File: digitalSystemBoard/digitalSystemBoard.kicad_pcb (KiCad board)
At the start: 2 copper layers, 180 x 130 mm, 200 parts, among them J1 Barrel_Jack, J10 Conn_02x03_Odd_Even, J11 Conn_02x03_Odd_Even, J12 Conn_02x03_Odd_Even, J2 USB-B, J3 Conn_02x04_Odd_Even, J4 Conn_02x04_Odd_Even, J5 Conn_02x08_Odd_Even, J6 Conn_02x07_Odd_Even, J7 Conn_02x07_Odd_Even, J8 Conn_02x08_Odd_Even, J9 Conn_02x03_Odd_Even, Q10 BC847, Q11 BC847, Q12 BC847, Q13 BC847, Q14 BC847, Q15 BC847, Q16 BC847, Q17 BC847, Q2 BC847, Q3 BC847, Q4 BC847, Q5 BC847, Q6 BC847, Q7 BC847, Q8 BC847, Q9 BC847, SW1 SW_SPDT, SW9 ButtonFirst, U10 IO_Switch, U11 IO_Switch, U12 IO_Switch, U13 IO_Switch, U14 74LS04, U15 Potentiometer, U16 ATmega32U4-AU, U17 ICSP, U18 74LS165, U19 74HC595, U2 KCSA02-105, U20 74LS165, U21 74HC595, U3 KCSA02-105, U4 74LS47, U5 74LS47, U6 IO_Switch, U7 IO_Switch, U8 IO_Switch, U9 IO_Switch, Y1 16MHz

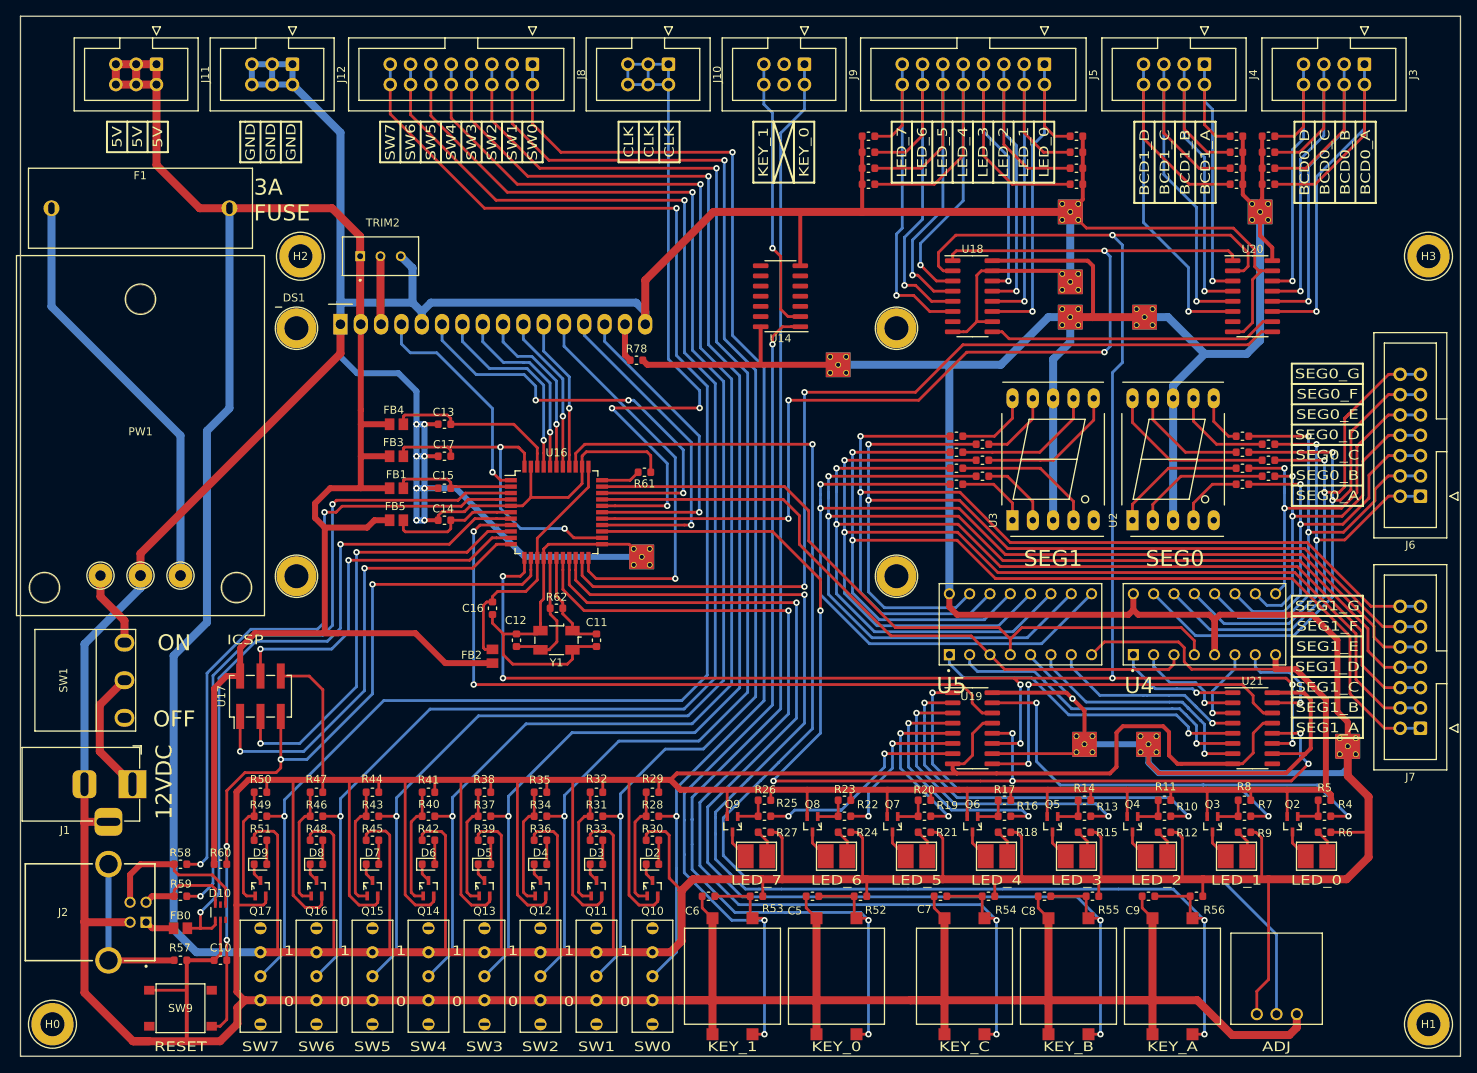
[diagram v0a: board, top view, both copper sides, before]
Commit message: Soldermask
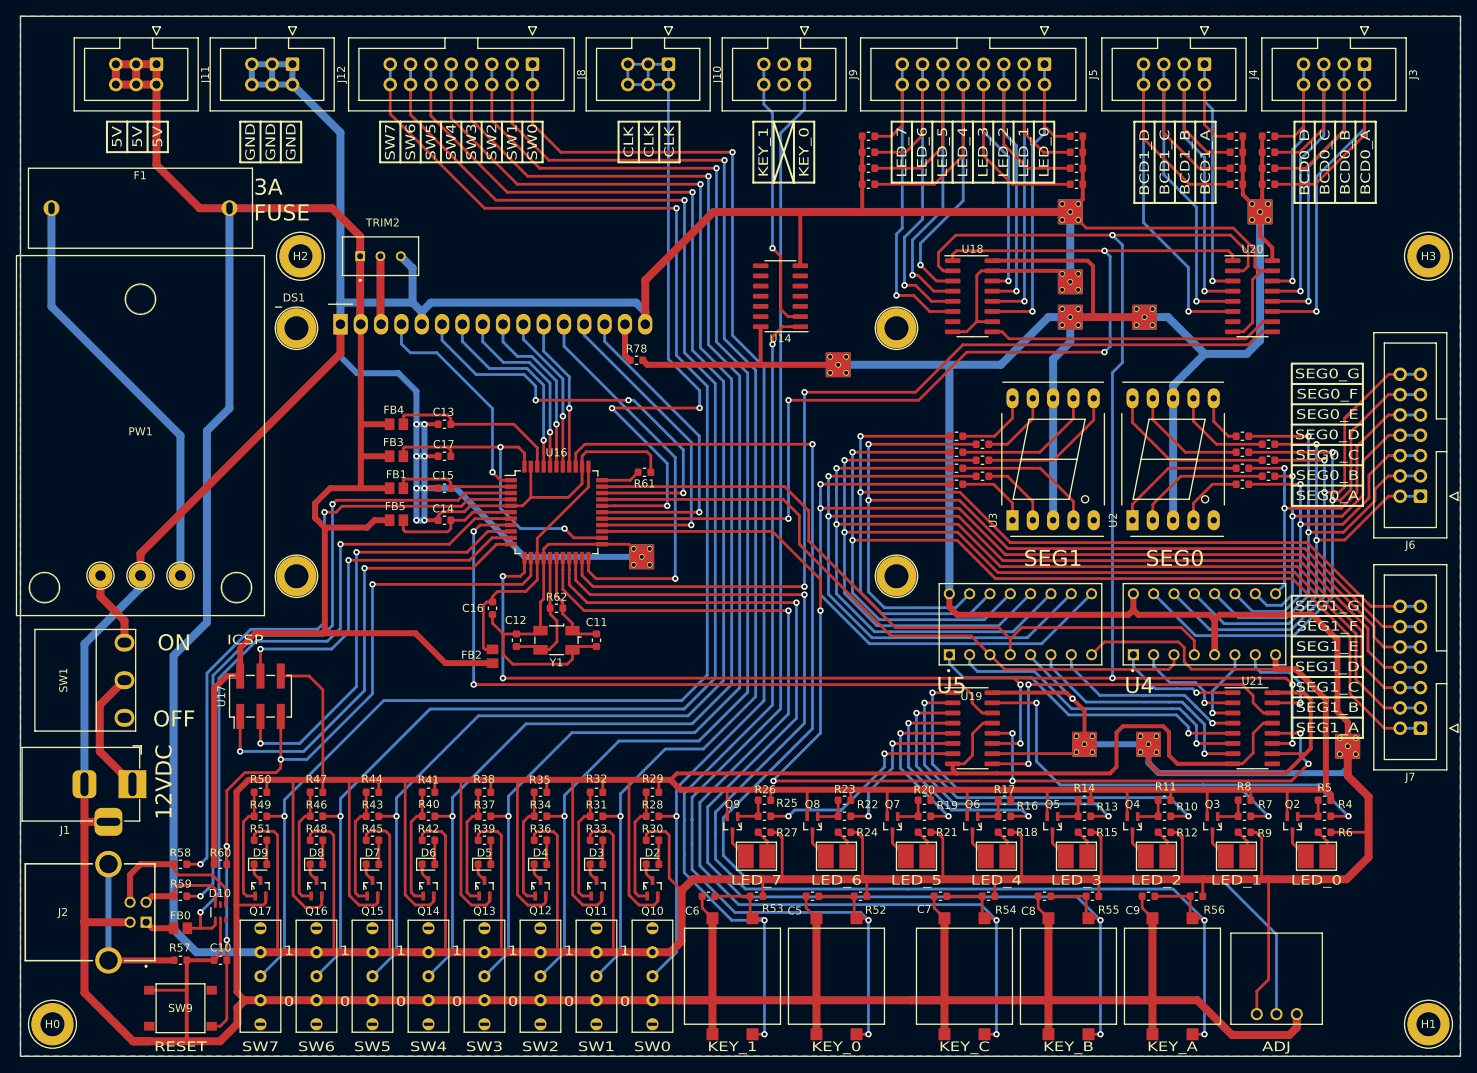
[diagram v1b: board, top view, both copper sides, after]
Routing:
- added copper zone on B.Cu, net GND
- added copper zone on F.Cu, net GND
